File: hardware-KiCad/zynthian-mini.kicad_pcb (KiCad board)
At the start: 2 copper layers, 165 x 108 mm, 39 parts, among them SW1 SW_Push, SW2 SW_Push, SW3 SW_Push, SW4 SW_Push, U1 74HCT14, U2 H11L1M

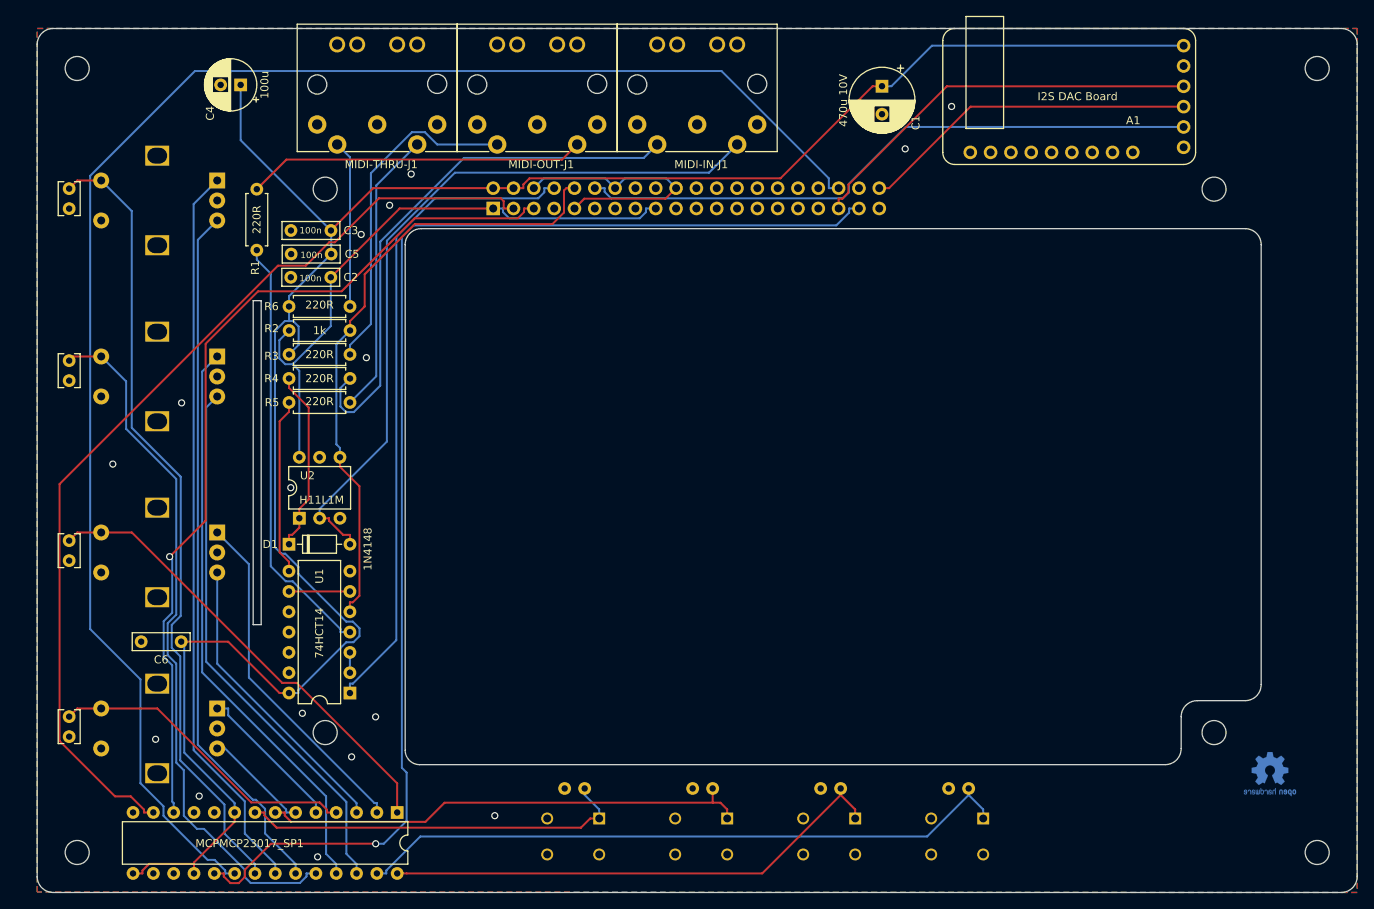
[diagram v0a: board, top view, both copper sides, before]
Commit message: reverted back to v1-beta version for saving it into its own branch
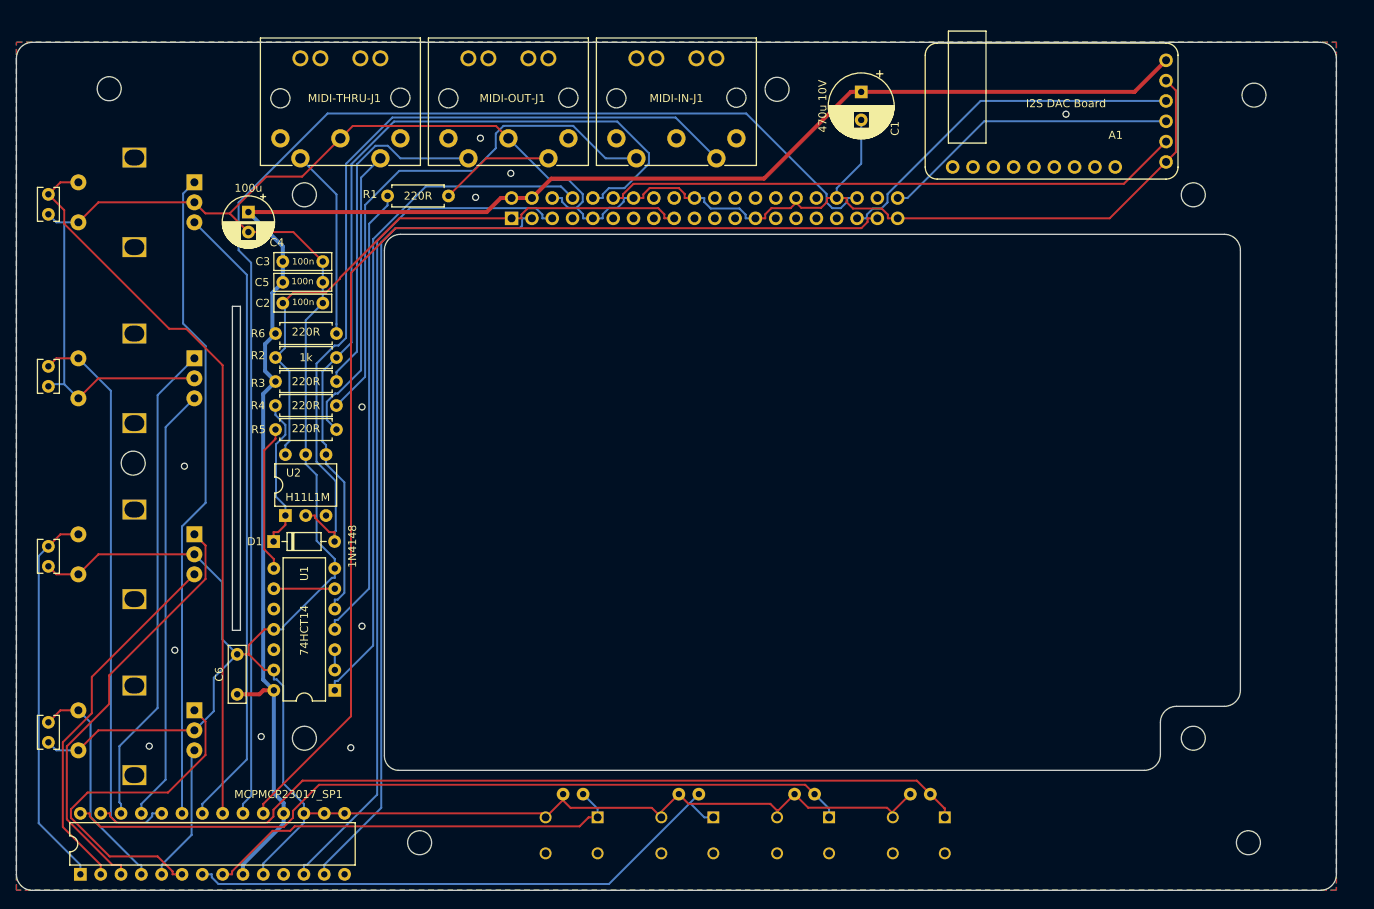
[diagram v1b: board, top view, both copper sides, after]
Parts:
- removed G***: MINI v2, project-footprints:Zynthian Logo Mask
- removed the REF** at (177.7, 117.2)
- added MINI v1.0: LOGO, My-Library:Zynthian Logo Mask, B.Cu at (162.0, 124.7)
- added REF**: OSHW-Logo2_7.3x6mm_SilkScreen, Symbol:OSHW-Logo2_7.3x6mm_SilkScreen, B.Cu at (176.4, 117.5)
- A1: footprint project-footprints:GY-PCM5102 -> clumsyMIDI:GY-PCM5102
- MIDI-IN-J1, MIDI-OUT-J1, MIDI-THRU-J1: footprint project-footprints:MultiDIN5 -> My-Library:MultiDIN5
- SW1, SW2, SW3, SW4: footprint project-footprints:push-button -> My-Library:push-button
- moved MCPMCP23017_SP1 40.3 mm to (29.0, 129.7), turned to 90 degrees
- moved R1 24.0 mm to (75.0, 44.9), turned to 180 degrees
- moved C4 15.9 mm to (50.0, 46.9), turned to -90 degrees
- moved C6 9.61 mm to (48.6, 107.2), turned to 90 degrees
- moved C3 7.16 mm to (54.3, 53.1), turned to 0 degrees
- moved C2 6.81 mm to (54.3, 58.3), turned to 0 degrees
- moved C5 5.30 mm to (59.3, 55.7), turned to 180 degrees
- moved MIDI-THRU-J1 4.91 mm to (54.0, 37.7)
- moved C31 4.85 mm to (135.2, 119.7)
- moved SW1 4.80 mm to (133.8, 124.8)
- moved MIDI-OUT-J1 3.99 mm to (75.0, 37.7)
- moved R2 3.78 mm to (53.4, 65.1)
- moved R4 3.78 mm to (61.0, 71.1)
- moved R3 3.78 mm to (53.4, 68.1)
- moved R6 3.78 mm to (53.4, 62.1)
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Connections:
- MCPMCP23017_SP1 pad 15: +5V -> GND
- MCPMCP23017_SP1 pad 2: ENC-A-3 -> ENC-B-3
- MCPMCP23017_SP1 pad 22: ENC-A-1 -> ENC-B-1
- MCPMCP23017_SP1 pad 23: ENC-B-1 -> ENC-A-1
- MCPMCP23017_SP1 pad 25: ENC-A-2 -> ENC-B-2
- MCPMCP23017_SP1 pad 26: ENC-B-2 -> ENC-A-2
- MCPMCP23017_SP1 pad 3: ENC-B-3 -> ENC-A-3
- MCPMCP23017_SP1 pad 5: ENC-A-4 -> ENC-B-4
- MCPMCP23017_SP1 pad 6: ENC-B-4 -> ENC-A-4
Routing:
- net GND: track 33.6 -> 489.3 mm, vias 16 -> 11
- net +5V: track 274.1 -> 217.5 mm
- net INTA: track 201.7 -> 165.7 mm
- net SWITCH-2: track 64.0 -> 99.5 mm
- net MIDI_IN: track 77.9 -> 110.3 mm
- net SWITCH-1: track 82.8 -> 111.5 mm
- net Net-(MIDI-OUT-J1-Pad5): track 42.4 -> 14.4 mm
- net ENC-A-4: track 18.9 -> 43.9 mm
- net INTB: track 160.6 -> 141.0 mm, vias 1 -> 0
- net SDA: track 120.4 -> 102.6 mm
- net ENC-SW-2: track 88.0 -> 70.5 mm
- net Net-(D1-Pad2): track 93.0 -> 106.7 mm
- net ENC-B-2: track 68.0 -> 54.6 mm
- net ENC-A-2: track 72.3 -> 60.8 mm
- net ENC-SW-4: track 39.4 -> 28.3 mm
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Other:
- board size 165 x 108 mm -> 165 x 106 mm

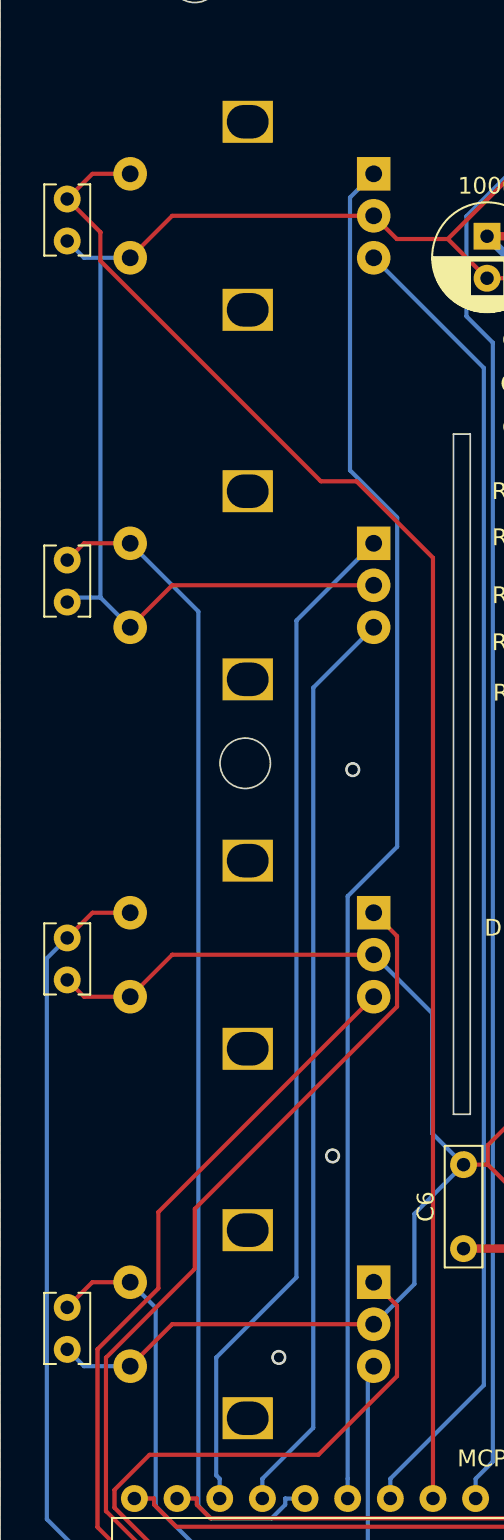
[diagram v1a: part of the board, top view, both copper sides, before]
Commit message: case almost completed - few fixes required
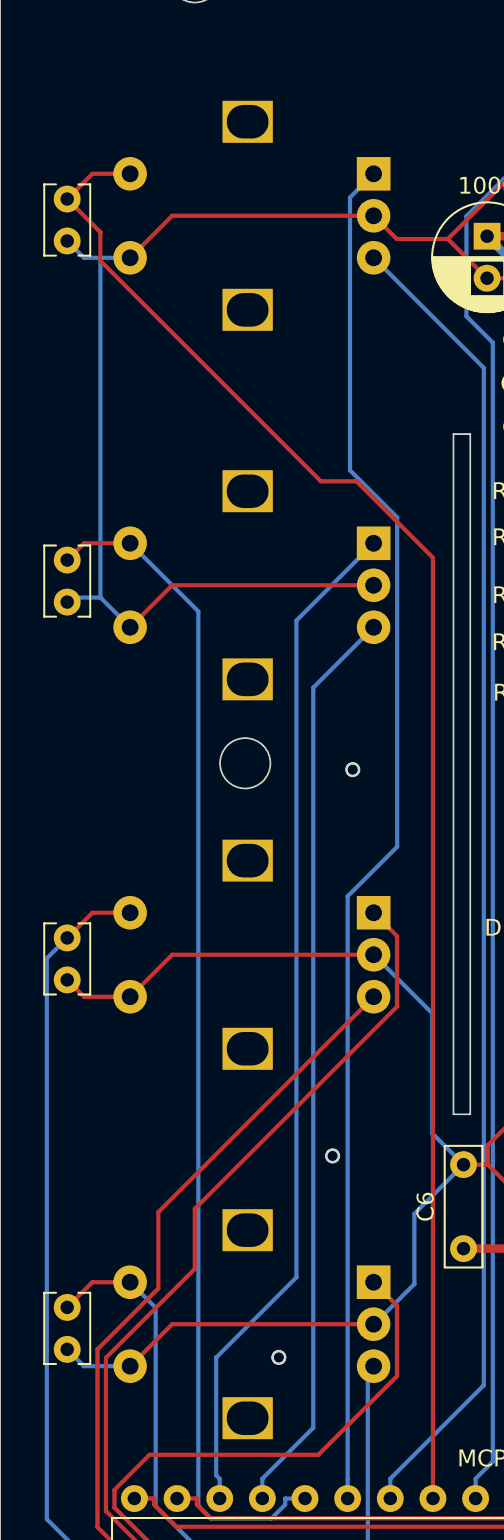
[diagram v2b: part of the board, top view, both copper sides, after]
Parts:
- Enc1, Enc2, Enc3, Enc4: footprint Rotary_Encoder:RotaryEncoder_Alps_EC12E-Switch_Vertical_H20mm -> project-footprints:RotaryEncoder_Alps_EC12E-Switch_Vertical_H20mm
- moved Enc1 7.91 mm to (35.8, 45.7)
- moved Enc2 7.91 mm to (35.8, 67.7)
- moved Enc3 7.91 mm to (35.8, 89.7)
- moved Enc4 7.91 mm to (35.8, 111.7)
